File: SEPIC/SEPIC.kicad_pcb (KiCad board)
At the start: 2 copper layers, 49 x 71.5 mm, 24 parts, among them J1 Screw Terminal, J2 Barrel Jack, J3 Pin Header, J4 Screw Terminal, Q1 IRF520N, U1 HCPL-3120

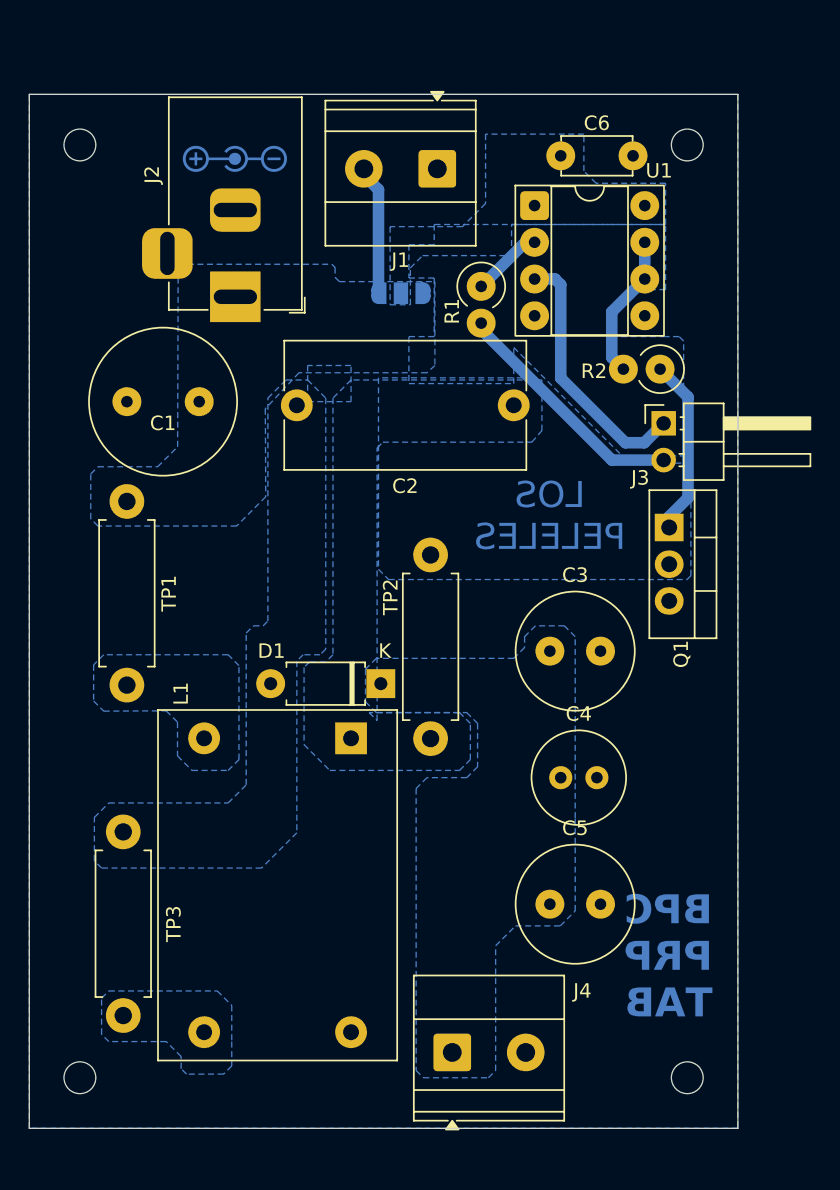
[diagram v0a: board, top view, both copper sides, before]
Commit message: PCB prototipo mejorado
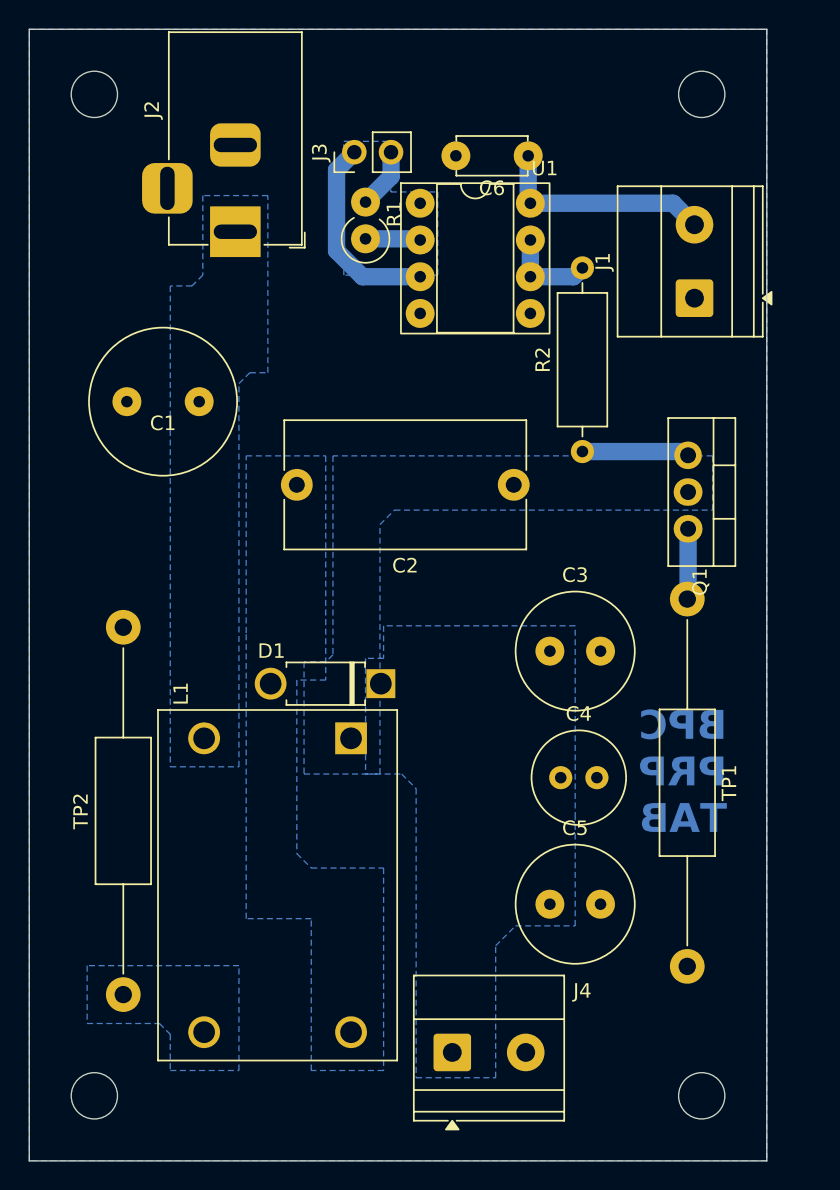
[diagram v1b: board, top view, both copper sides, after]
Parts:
- removed JP1: Solder Jumper, Jumper:SolderJumper-3_P1.3mm_Open_RoundedPad1.0x1.5mm
- removed the REF** at (39.8, 29.8)
- removed the REF** at (81.8, 29.8)
- removed the REF** at (39.8, 94.2)
- removed the REF** at (81.8, 94.2)
- removed the TP1 at (43.0, 54.4)
- added REF**: MountingHole_3.2mm_M3, MountingHole:MountingHole_3.2mm_M3, F.Cu at (40.8, 95.5)
- added REF**: MountingHole_3.2mm_M3, MountingHole:MountingHole_3.2mm_M3, F.Cu at (82.8, 95.5)
- added REF**: MountingHole_3.2mm_M3, MountingHole:MountingHole_3.2mm_M3, F.Cu at (40.8, 26.2)
- added REF**: MountingHole_3.2mm_M3, MountingHole:MountingHole_3.2mm_M3, F.Cu at (82.8, 26.2)
- J3: footprint Connector_PinHeader_2.54mm:PinHeader_1x02_P2.54mm_Horizontal -> Connector_PinHeader_2.54mm:PinHeader_1x02_P2.54mm_Vertical
- L1: value 3m -> 2m
- R2: footprint Resistor_THT:R_Axial_DIN0309_L9.0mm_D3.2mm_P2.54mm_Vertical -> Resistor_THT:R_Axial_DIN0309_L9.0mm_D3.2mm_P12.70mm_Horizontal
- TP1: renamed from TP2; footprint Resistor_THT:R_Axial_DIN0411_L9.9mm_D3.6mm_P12.70mm_Horizontal -> Resistor_THT:R_Axial_DIN0411_L9.9mm_D3.6mm_P25.40mm_Horizontal
- TP2: renamed from TP3; footprint Resistor_THT:R_Axial_DIN0411_L9.9mm_D3.6mm_P12.70mm_Horizontal -> Resistor_THT:R_Axial_DIN0411_L9.9mm_D3.6mm_P25.40mm_Horizontal
- moved J3 28.4 mm to (58.7, 30.2), turned to 90 degrees
- moved TP1 20.2 mm to (81.8, 61.1), turned to -90 degrees
- moved J1 19.9 mm to (82.2, 40.3), turned to 90 degrees
- moved TP2 11.2 mm to (42.8, 88.5), turned to 90 degrees
- moved R1 8.65 mm to (59.5, 36.2), turned to 90 degrees
- moved U1 7.91 mm to (63.3, 33.8)
- moved R2 7.83 mm to (74.5, 51.0), turned to 90 degrees
- moved C2 5.50 mm to (69.8, 53.2)
- moved Q1 5.16 mm to (81.8, 51.2)
- moved J2 4.50 mm to (50.5, 35.8)
- moved C6 2.25 mm to (70.8, 30.5), turned to 180 degrees
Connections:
- C2 pad 1: Net-(C2-Pad1) -> Net-(Q1-D)
- J1 pad 2: Net-(J1-Pin_2) -> VCC
- J2 pad 3: (no net) -> unconnected-(J2-MountPin-Pad3)
- L1 pad 1: Net-(C2-Pad1) -> Net-(Q1-D)
- L1 pad 2: Net-(L1-Pad2) -> +24V
- L1 pad 4: GND -> Net-(D1-A)
- Q1 pad 3: GND -> Net-(Q1-S)
- TP1 pad 1: Net-(C2-Pad1) -> Net-(Q1-S)
- TP1 pad 2: Net-(Q1-D) -> GND
- TP2 pad 1: Net-(D1-A) -> Net-(L1-Pad3)
- TP2 pad 2: Net-(L1-Pad3) -> GND
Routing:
- net VCC: track 0.00 -> 15.3 mm
- net Net-(J3-Pin_2): track 16.8 -> 4.18 mm
- net Net-(J1-Pin_2): track 8.59 -> 0.00 mm
- net Net-(Q1-S): track 0.00 -> 4.88 mm
- net PWM: track 12.3 -> 7.41 mm
- net Net-(J3-Pin_1): track 17.9 -> 13.8 mm
- net Net-(R2-Pad2): track 10.0 -> 6.39 mm
- net Net-(U1-A): track 4.95 -> 3.61 mm
- removed copper zone on B.Cu, net Net-(C2-Pad1)
- removed copper zone on B.Cu, net Net-(L1-Pad2)
- removed copper zone on B.Cu, net VCC
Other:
- board size 49 x 71.5 mm -> 51 x 78.2 mm
- board text removed: "LOS PELELES"
